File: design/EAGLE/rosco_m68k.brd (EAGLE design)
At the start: 160 x 100 mm, 74 parts, among them IC1 74LS04N, IC10 74LS32N, IC11 NE555N, IC12 74LS01N, IC2 MC68010P10, IC3 ATF16V8QL-15PU, IC4 74LS93N, IC5 74S20N, IC6 MC68901P, IC7 74LS08N, IC8 74LS08N, IC9 74LS174N, Q1 1.8432MHz, Q2 8MHz, U1 AT28C64B-15PU, U2 AT28C64B-15PU, U3 AS6C4008-55PCN, U4 AS6C4008-55PCN

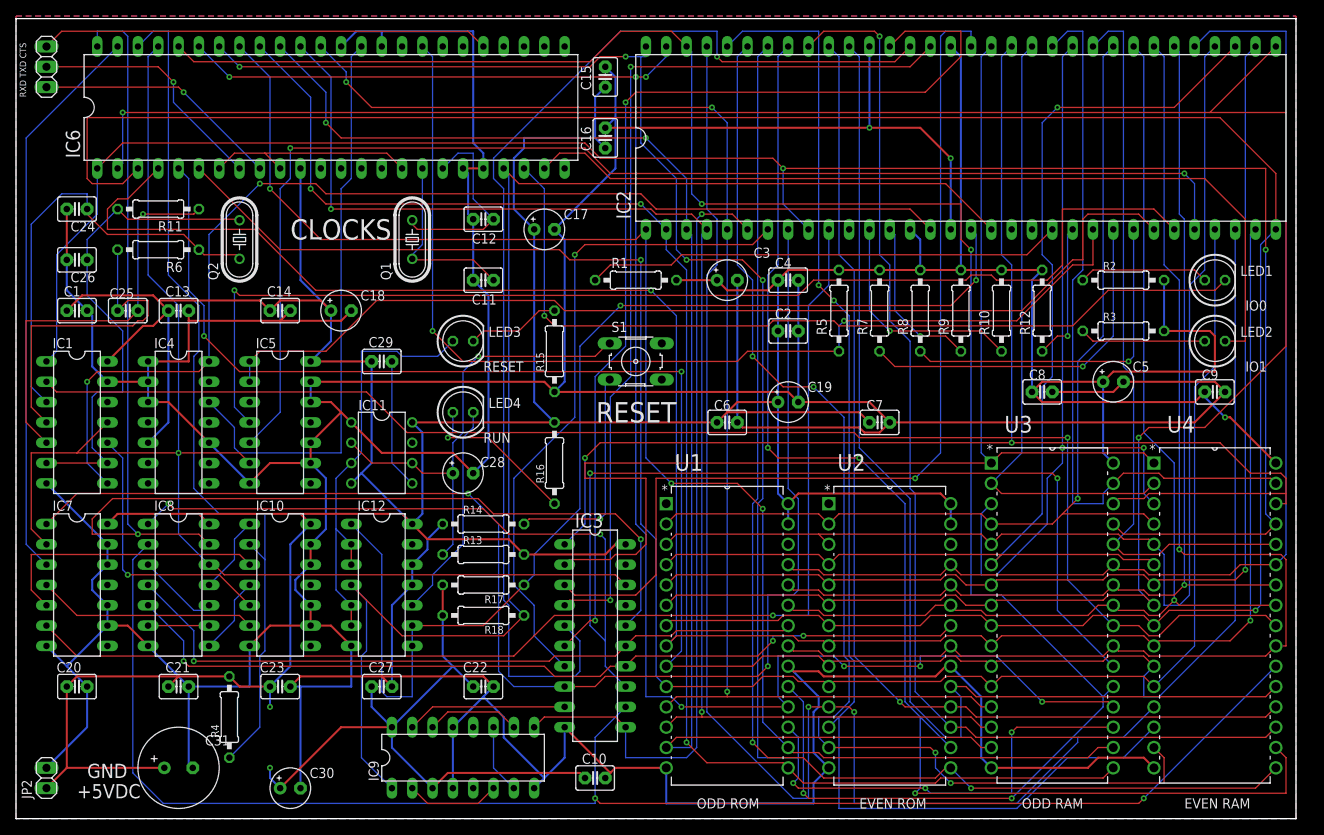
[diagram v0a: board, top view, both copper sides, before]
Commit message: New PCB design
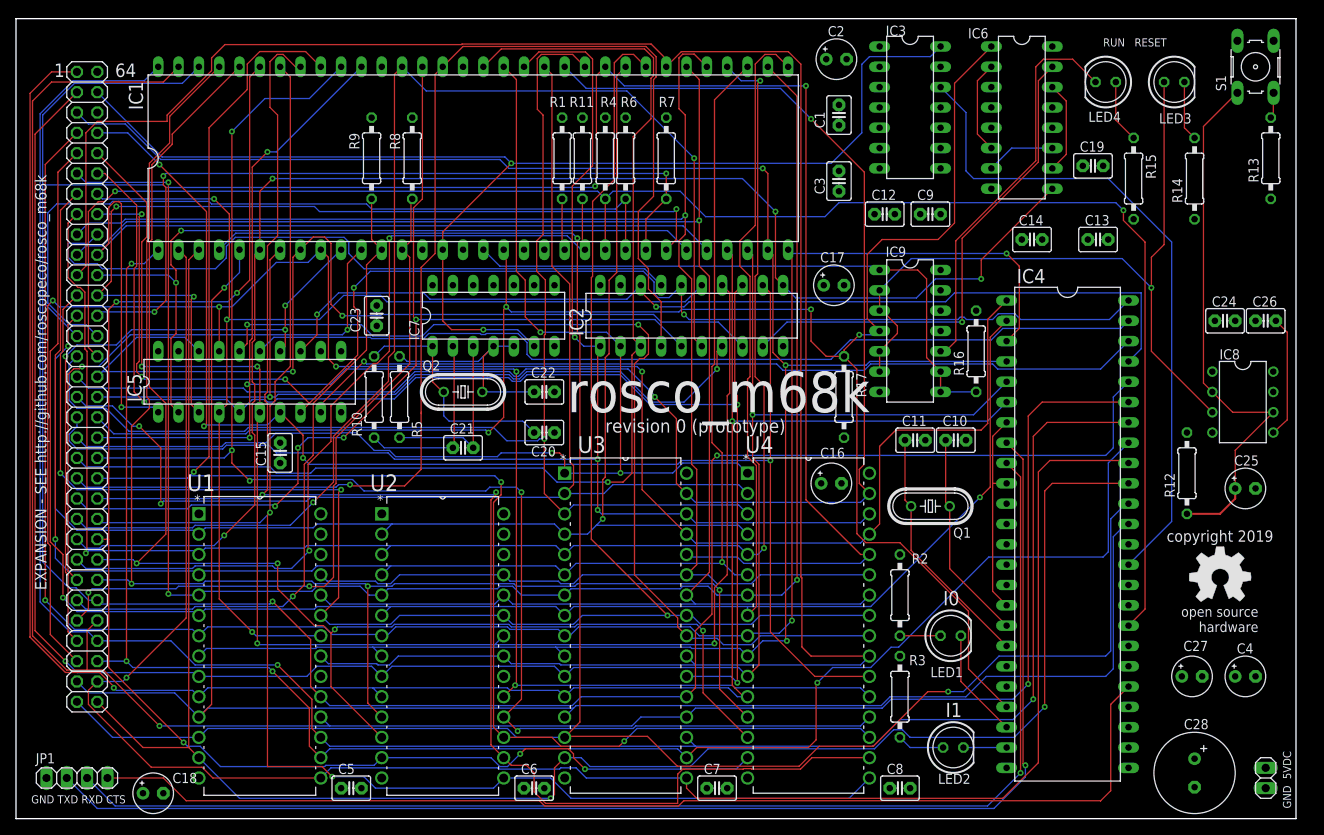
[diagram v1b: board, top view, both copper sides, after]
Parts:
- removed C29: 100nF, capacitor-wima:C2.5-3
- removed C30: 100uF, rcl:E2,5-5
- removed C31: 400uF, rcl:E3,5-10
- removed IC10: 74LS32N, 74xx-eu:DIL14
- removed IC11: NE555N, linear:DIL08
- removed IC12: 74LS01N, 74xx-eu:DIL14
- removed R18: 4K7, rcl:0207/10
- added JP3: (no value), pinhead:2X30
- added JP4: (no value), pinhead:2X02
- added U$1: (no value), oshw:OSHW_8MM
- C10: value 100nF -> 33pF
- C12: value 33pF -> 100nF
- C16, C2, C25, C27, C4: value 100nF -> 100uF; device capacitor-wima:C2.5-3 -> rcl:E2,5-5
- C19, C3, C5: value 100uF -> 100nF; device rcl:E2,5-5 -> capacitor-wima:C2.5-3
- C20, C22: value 100nF -> 22pF
- C24, C26: value 22pF -> 100nF
- C28: value 100uF -> 400uF; device rcl:E2,5-5 -> rcl:E3,5-10
- IC1: value 74LS04N -> MC68010P10; device 74xx-eu:DIL14 -> micro-mc68000:DIL64
- IC2: value MC68010P10 -> ATF16V8QL-15PU; device micro-mc68000:DIL64 -> atmel:DIL20
- IC3: value ATF16V8QL-15PU -> 74LS93N; device atmel:DIL20 -> 74xx-eu:DIL14
- IC4: value 74LS93N -> MC68901P; device 74xx-eu:DIL14 -> micro-mc68000:DIL48
- IC5: value 74S20N -> ATF16V8QL-15PU; device 74xx-eu:DIL14 -> atmel:DIL20
- IC6: value MC68901P -> 74LS174N; device micro-mc68000:DIL48 -> 74xx-eu:DIL16
- IC7: value 74LS08N -> 74LS04N
- IC8: value 74LS08N -> NE555N; device 74xx-eu:DIL14 -> linear:DIL08
- IC9: value 74LS174N -> 74LS01N; device 74xx-eu:DIL16 -> 74xx-eu:DIL14
- JP1: device pinhead:1X03 -> pinhead:1X04
- R10, R5: value 4K7 -> 1K2
- R11, R6: value 1K2 -> 4K7
- R12: value 4K7 -> 2K2
- R13: value 2K2 -> 270R
- R14: value 270R -> 330R
- R16: value 330R -> 4K7
- moved JP2 152.4 mm to (156.2, 5.08), turned to 270 degrees
- moved C26 148.8 mm to (156.2, 62.2), turned to 0 degrees
- moved C24 144.2 mm to (151.1, 62.2), turned to 0 degrees
- moved C25 141.5 mm to (153.7, 41.3)
- moved IC8 135.0 mm to (153.4, 52.1)
- moved C13 115.3 mm to (135.3, 72.4)
- moved IC4 112.0 mm to (131.4, 35.6)
- moved R13 110.2 mm to (156.8, 82.5), turned to 90 degrees
- moved C5 108.0 mm to (41.9, 3.81)
- moved C27 101.3 mm to (147.0, 17.8)
- moved R14 98.8 mm to (147.3, 80.0), turned to 90 degrees
- moved C28 98.8 mm to (147.3, 5.71), turned to 270 degrees
- moved C1 98.3 mm to (102.9, 87.9), turned to 90 degrees
- moved LED3 94.6 mm to (144.8, 92.1)
- moved C14 94.4 mm to (127.0, 72.4)
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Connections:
- removed net IACK: IC1.10, IC10.5
- removed net N$11: IC6.10, IC6.16, IC6.7
- removed net N$12: IC6.22, LED1.K
- removed net N$13: IC6.9, JP1.1
- removed net N$14: IC6.8, JP1.2
- removed net N$15: IC8.6, IC8.9
- removed net N$17: IC6.23, LED2.K
- removed net N$18: IC6.29, JP1.3
- removed net N$2: IC2.21, R1.1
- removed net N$24: IC8.10, IC8.3
- removed net N$25: IC10.4, IC8.8
- removed net N$27: IC10.1, IC8.11
- removed net N$28: IC10.6, IC7.4
- removed net N$29: IC10.3, IC7.5
- removed net N$7: C11.1, IC6.17, Q1.1
- removed net N$8: C12.1, IC6.18, Q1.2
- new net MFPIO0: IC4.22, LED1.K
- new net MFPIO1: IC4.23, LED2.K
- new net MFPXTAL1: C10.1, IC4.17, Q1.1
- new net MFPXTAL2: C11.1, IC4.18, Q1.2
- new net UARTCLK: IC4.10, IC4.16, IC4.7
- new net UARTCTS: IC4.29, JP1.4
- new net UARTRX: IC4.9, JP1.3
- new net UARTTX: IC4.8, JP1.2
- new net VPA: IC1.21, R1.1
- net /BOOT: now also IC2.9, IC6.15; no longer IC3.9, IC9.15
- net /HALT: now also IC1.17, IC9.1, IC9.8, IC9.9, R16.1; no longer IC12.1, IC12.8, IC12.9, IC2.17, R17.1
- net /IACK: now also IC2.18, IC4.45, IC5.13; no longer IC1.11, IC3.18, IC5.6, IC6.45, IC7.2, IC8.12
- net /IODTACK: now also IC4.46, IC5.9; no longer IC10.2, IC6.46, R4.1
- net /MFPDS: now also IC4.47, IC5.15; no longer IC6.47, IC7.3
- net /RAMOE: now also IC5.16; no longer IC1.2
- net A1: now also IC1.29, IC4.6, JP3.1; no longer IC2.29, IC6.6
- net A10: now also IC1.38, JP3.19; no longer IC2.38
- net A11: now also IC1.39, JP3.21; no longer IC2.39
- net A12: now also IC1.40, JP3.23; no longer IC2.40
- net A13: now also IC1.41, JP3.25; no longer IC2.41
- net A14: now also IC1.42, JP3.27; no longer IC2.42
- net A15: now also IC1.43, JP3.29; no longer IC2.43
- net A16: now also IC1.44, JP3.31; no longer IC2.44
- net A17: now also IC1.45, JP3.33; no longer IC2.45
- net A18: now also IC1.46, IC2.1, JP3.35; no longer IC2.46, IC3.1
- net A19: now also IC1.47, IC2.2, JP3.37; no longer IC2.47, IC3.2
- net A2: now also IC1.30, IC4.5, JP3.3; no longer IC2.30, IC6.5
- net A20: now also IC1.48, IC2.3, JP3.39; no longer IC2.48, IC3.3
- net A21: now also IC1.50, IC2.4, JP3.41; no longer IC2.50, IC3.4
- net A22: now also IC1.51, IC2.5, JP3.43; no longer IC2.51, IC3.5
- net A23: now also IC1.52, IC2.6, JP3.45; no longer IC2.52, IC3.6
- net A3: now also IC1.31, IC4.4, JP3.5; no longer IC2.31, IC6.4
- net A4: now also IC1.32, IC4.3, JP3.7; no longer IC2.32, IC6.3
- net A5: now also IC1.33, IC4.2, JP3.9; no longer IC2.33, IC6.2
- net A6: now also IC1.34, JP3.11; no longer IC2.34
- net A7: now also IC1.35, JP3.13; no longer IC2.35
- net A8: now also IC1.36, JP3.15; no longer IC2.36
- net A9: now also IC1.37, JP3.17; no longer IC2.37
- net AS: now also IC1.6, IC2.11, IC6.9, JP3.47; no longer IC2.6, IC3.11, IC9.9
- net BERR: now also IC1.22, JP3.49, R11.1; no longer IC2.22, R12.1
- net BG: now also IC1.11, JP3.51; no longer IC2.11
- net BGACK: now also IC1.12, JP3.53, R9.1; no longer IC2.12, R10.1
- net BR: now also IC1.13, JP3.55, R8.1; no longer IC2.13, R9.1
- net CLK: now also IC1.15, IC3.14, IC7.6, JP3.4; no longer IC1.8, IC2.15, IC4.14
- net D0: now also IC1.5, IC4.37, JP4.1; no longer IC2.5, IC6.37
- net D1: now also IC1.4, IC4.38, JP4.3; no longer IC2.4, IC6.38
- net D10: now also IC1.59, JP3.48; no longer IC2.59
- net D11: now also IC1.58, JP3.46; no longer IC2.58
- net D12: now also IC1.57, JP3.44; no longer IC2.57
- net D13: now also IC1.56, JP3.42; no longer IC2.56
- net D14: now also IC1.55, JP3.40; no longer IC2.55
- net D15: now also IC1.54, JP3.38; no longer IC2.54
- net D2: now also IC1.3, IC4.39, JP4.4; no longer IC2.3, IC6.39
- net D3: now also IC1.2, IC4.40, JP4.2; no longer IC2.2, IC6.40
- net D4: now also IC1.1, IC4.41, JP3.60; no longer IC2.1, IC6.41
- net D5: now also IC1.64, IC4.42, JP3.58; no longer IC2.64, IC6.42
- net D6: now also IC1.63, IC4.43, JP3.56; no longer IC2.63, IC6.43
- net D7: now also IC1.62, IC4.44, JP3.54; no longer IC2.62, IC6.44
- net D8: now also IC1.61, JP3.52; no longer IC2.61
- net D9: now also IC1.60, JP3.50; no longer IC2.60
- net DTACK: now also IC1.10, IC5.14, JP3.57; no longer IC2.10, IC7.6
- net EVENRAMSEL: now also IC2.12, IC5.7, JP3.8; no longer IC3.12, IC8.2
- net EVENROMSEL: now also IC2.14, IC5.6, JP3.10; no longer IC3.14, IC8.5
- net EXPSEL: now also IC2.17, JP3.18; no longer IC3.17
- net FC0: now also IC1.28, IC5.1, JP3.20; no longer IC2.28, IC5.5
- net FC1: now also IC1.27, IC5.2, JP3.22; no longer IC2.27, IC5.4
- net FC2: now also IC1.26, IC5.3, JP3.24; no longer IC2.26, IC5.1, IC5.2
- net GND: now also C16.-, C19.2, C2.-, C25.-, C27.-, C3.2, C4.-, C5.2, IC1.16, IC1.53, IC2.10, IC3.1, IC3.2, IC3.3, IC4.19, IC4.20, IC4.34, IC4.36, IC5.11, IC6.13, IC6.4, IC6.8, IC7.11, IC8.1, IC9.11, IC9.12, IC9.7, JP1.1, JP3.6, R13.1; no longer C16.2, C19.-, C2.2, C21.2, C26.2, C27.2, C3.-, C30.-, C31.-, C4.2, C5.-, IC1.13, IC1.7, IC10.10, IC10.12, IC10.13, IC10.7, IC10.9, IC11.1, IC12.11, IC12.12, IC12.7, IC2.16, IC2.53, IC4.1, IC4.10, IC4.2, IC4.3, IC5.12, IC5.13, IC5.7, IC5.9, IC6.19, IC6.20, IC6.34, IC6.36, IC7.10, IC7.12, IC8.7, IC9.13, IC9.4, IC9.8, R15.1
- net IOSEL: now also IC2.16, IC4.48, IC5.8, JP3.16; no longer IC3.16, IC6.48, IC8.13
- net IPL0: now also IC1.25, JP3.26, R7.1; no longer IC2.25, R8.1
- net IPL1: now also IC1.24, JP3.28, R6.1; no longer IC2.24, R7.1
- net IPL2: now also IC1.23, IC4.32, JP3.30, R4.1; no longer IC2.23, IC6.32, R5.1
- net LDS: now also IC1.8, IC5.18, JP3.32; no longer IC3.8, IC7.1
- net MFPCLK: now also IC3.12, IC4.35; no longer IC4.12, IC6.35
- net N$16: now also IC6.11, IC6.7; no longer IC9.11, IC9.7
- net N$19: now also C26.2, IC8.5; no longer C29.2, IC11.5
- net N$20: now also R14.2; no longer R15.2
- net N$22: now also IC6.10, IC6.14; no longer IC9.10, IC9.14
- net N$23: now also IC6.2, IC6.6; no longer IC9.2, IC9.6
- net N$3: now also C21.1, IC7.2, R5.2; no longer C25.1, IC1.4, R6.2
- net N$33: now also IC9.10; no longer IC12.10
- net N$34: now also R15.1; no longer R16.1
- net N$35: now also IC8.3, IC9.2, IC9.3, IC9.5, IC9.6; no longer IC11.3, IC12.2, IC12.3, IC12.5, IC12.6
- net N$36: now also R13.2; no longer R14.2
- net N$37: now also C25.+, IC8.2, IC8.6, R12.1; no longer C28.+, IC11.2, IC11.6, R13.1
- net N$4: now also C21.2, IC7.3, R10.1; no longer C25.2, IC1.5, R11.1
- net N$5: now also C22.1, IC7.4, IC7.5, R10.2; no longer C26.1, IC1.6, IC1.9, R11.2
- net N$6: now also C20.1, IC7.1, R5.1; no longer C24.1, IC1.3, R6.1
- net ODDRAMSEL: now also IC2.13, IC5.5, JP3.12; no longer IC3.13, IC8.1
- net ODDROMSEL: now also IC2.15, IC5.4, JP3.14; no longer IC3.15, IC8.4
- net R/W: now also IC1.9, IC4.1, IC5.17, JP3.59; no longer IC1.1, IC2.9, IC6.1
- net RESET: now also IC1.18, IC4.21, IC6.1, IC9.4, JP3.36, R17.1; no longer IC12.4, IC2.18, IC6.21, IC9.1, R18.1
- net UDS: now also IC1.7, JP3.34; no longer IC3.7
- net VCC: now also C12.1, C16.+, C19.1, C2.+, C24.1, C26.1, C27.+, C28.+, C3.1, C4.+, C5.1, IC1.49, IC2.20, IC3.5, IC4.11, IC5.20, IC6.16, IC6.3, IC8.4, IC8.8, IC9.14, JP3.2, R11.2, R15.2, R6.2; no longer C10.1, C16.1, C19.+, C2.1, C20.1, C21.1, C22.1, C27.1, C29.1, C3.+, C30.+, C31.+, C4.1, C5.+, IC10.14, IC11.4, IC11.8, IC12.14, IC2.14, IC2.49, IC3.20, IC4.5, IC5.14, IC6.11, IC8.14, IC9.16, IC9.3, R10.2, R13.2, R18.2, R5.2
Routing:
- net GND: track 867.3 -> 0.00 mm, vias 2 -> 0
- net VCC: track 731.0 -> 0.00 mm, vias 3 -> 0
- net UARTTX: track 0.00 -> 165.9 mm, vias 0 -> 1
- net UARTRX: track 0.00 -> 159.3 mm, vias 0 -> 1
- net UARTCTS: track 0.00 -> 141.6 mm
- net A14: track 91.7 -> 217.3 mm, vias 0 -> 2
- net A11: track 154.2 -> 270.6 mm, vias 1 -> 0
- net N$17: track 109.6 -> 0.00 mm
- net N$12: track 108.0 -> 0.00 mm, vias 1 -> 0
- net A16: track 92.4 -> 197.6 mm, vias 0 -> 2
- net D1: track 172.9 -> 268.1 mm
- net A12: track 136.0 -> 226.4 mm, vias 1 -> 3
- net BERR: track 17.6 -> 106.1 mm, vias 1 -> 2
- net A10: track 132.0 -> 220.0 mm
- net EXPSEL: track 0.00 -> 86.4 mm
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- added copper zone on layer 2, net GND
- added copper zone on layer 15, net VCC
- removed copper zone on layer 16, net GND
- removed copper zone on layer 1, net VCC
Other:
- board text added: "1"
- board text added: "64"
- board text added: "EXPANSION - SEE http://github.com/roscopeco/rosco_m68k"
- board text added: "GND 5VDC"
- board text added: "GND TXD RXD CTS"
- board text added: "I0"
- board text added: "I1"
- board text added: "RUN RESET"
- board text added: "copyright 2019"
- board text added: "revision 0 (prototype)"
- board text added: "rosco_m68k revision zero"
- board text removed: "(c)2019"
- board text removed: "+5VDC"
- board text removed: "CLOCKS"
- board text removed: "EVEN RAM"
- board text removed: "EVEN ROM"
- board text removed: "GND"
- board text removed: "IO0"
- board text removed: "IO1"
- board text removed: "ODD RAM"
- board text removed: "ODD ROM"
- board text removed: "RESET"
- board text removed: "RUN"
- board text removed: "RXD TXD CTS"
- board text removed: "Version 1r0 (Prototype)"
- board text removed: "http://github.com/roscopeco/rosco_m68k"
